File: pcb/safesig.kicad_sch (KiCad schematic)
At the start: 6 parts, among them U7 74HC123

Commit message: Add LCSCs.
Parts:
- R27, R28: LCSC (none) -> C17713
- U7: LCSC (none) -> C91435
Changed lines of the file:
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@@
+      (effects (font (size 1.27 1.27)) hide)
+    )
+    (property "LCSC" "C91435" (id 4) (at 92.075 65.405 0)
       (effects (font (size 1.27 1.27)) hide)
     )
@@
       (effects (font (size 1.27 1.27)) hide)
     )
+    (property "LCSC" "C91435" (id 4) (at 92.075 120.65 0)
+      (effects (font (size 1.27 1.27)) hide)
+    )
     (pin "1")
     (pin "13")
@@
       (effects (font (size 1.27 1.27)) hide)
     )
+    (property "LCSC" "C17713" (id 4) (at 69.85 49.53 0)
+      (effects (font (size 1.27 1.27)) hide)
+    )
     (pin "1")
     (pin "2")
@@
       (effects (font (size 1.27 1.27)) hide)
     )
+    (property "LCSC" "C17713" (id 4) (at 69.85 104.775 0)
+      (effects (font (size 1.27 1.27)) hide)
+    )
     (pin "1")
     (pin "2")
@@
       (effects (font (size 1.27 1.27)) hide)
     )
+    (property "LCSC" "C91435" (id 4) (at 231.14 91.44 0)
+      (effects (font (size 1.27 1.27)) hide)
+    )

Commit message: Tweak silkscreen.
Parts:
- U7: JLCPCB_CORRECTION (none) -> 0;0;270
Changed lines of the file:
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@@
+      (effects (font (size 1.27 1.27)) hide)
+    )
+    (property "JLCPCB_CORRECTION" "0;0;270" (id 5) (at 92.075 65.405 0)
       (effects (font (size 1.27 1.27)) hide)
     )
@@
       (effects (font (size 1.27 1.27)) hide)
     )
+    (property "JLCPCB_CORRECTION" "0;0;270" (id 5) (at 92.075 120.65 0)
+      (effects (font (size 1.27 1.27)) hide)
+    )
     (pin "1")
     (pin "13")
@@
       (effects (font (size 1.27 1.27)) hide)
     )
+    (property "JLCPCB_CORRECTION" "0;0;270" (id 5) (at 231.14 91.44 0)
+      (effects (font (size 1.27 1.27)) hide)
+    )

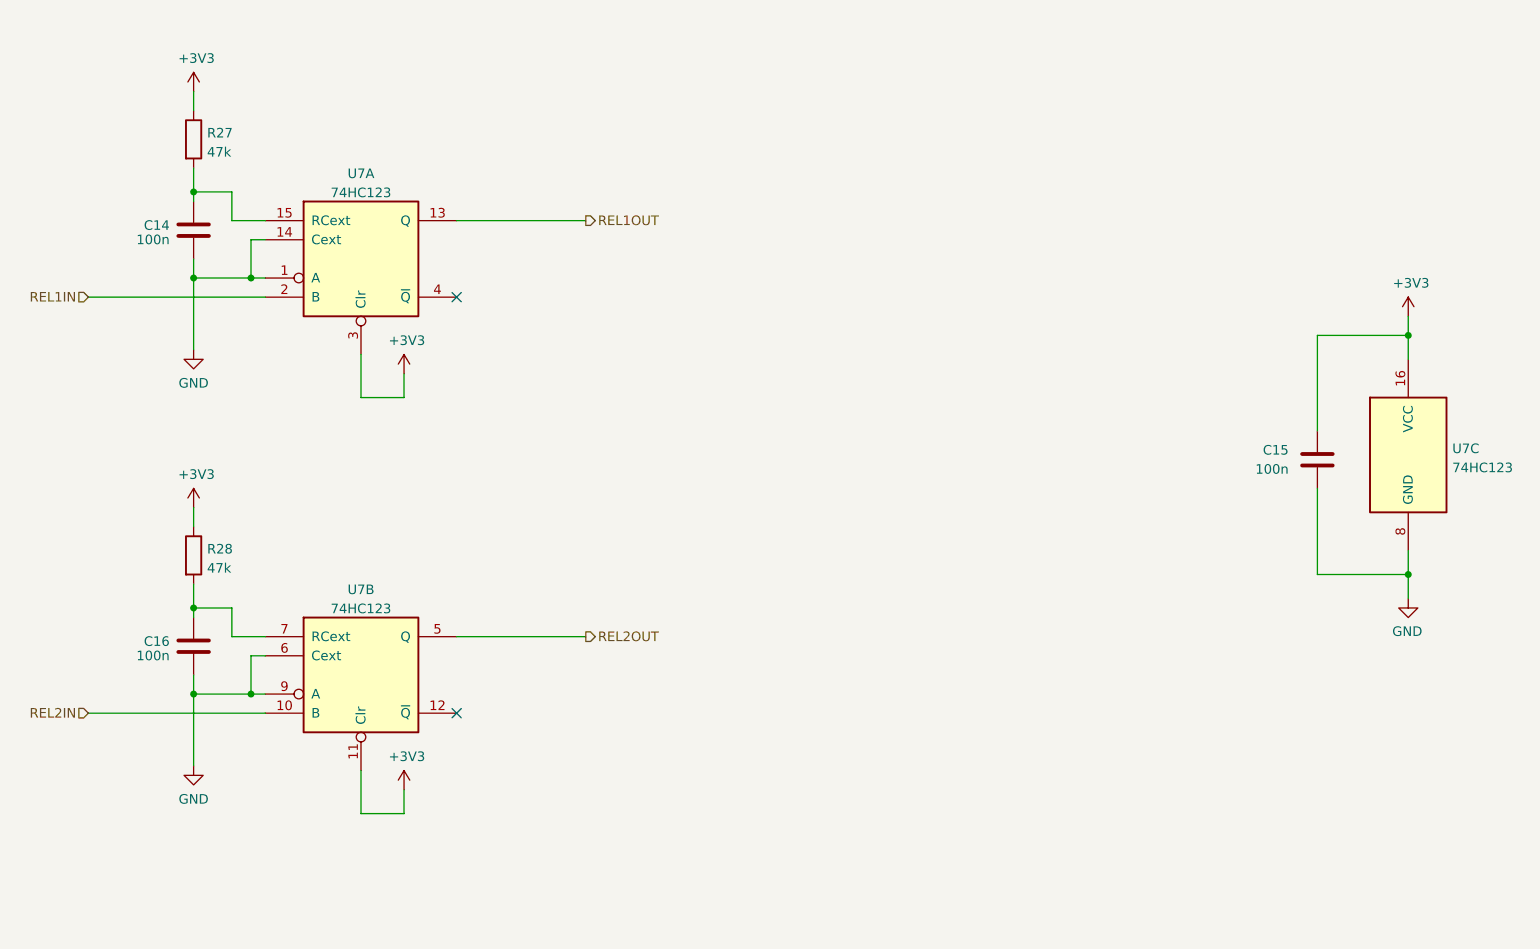
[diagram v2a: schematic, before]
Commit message: Add pull-down resistors to relay logic signals.
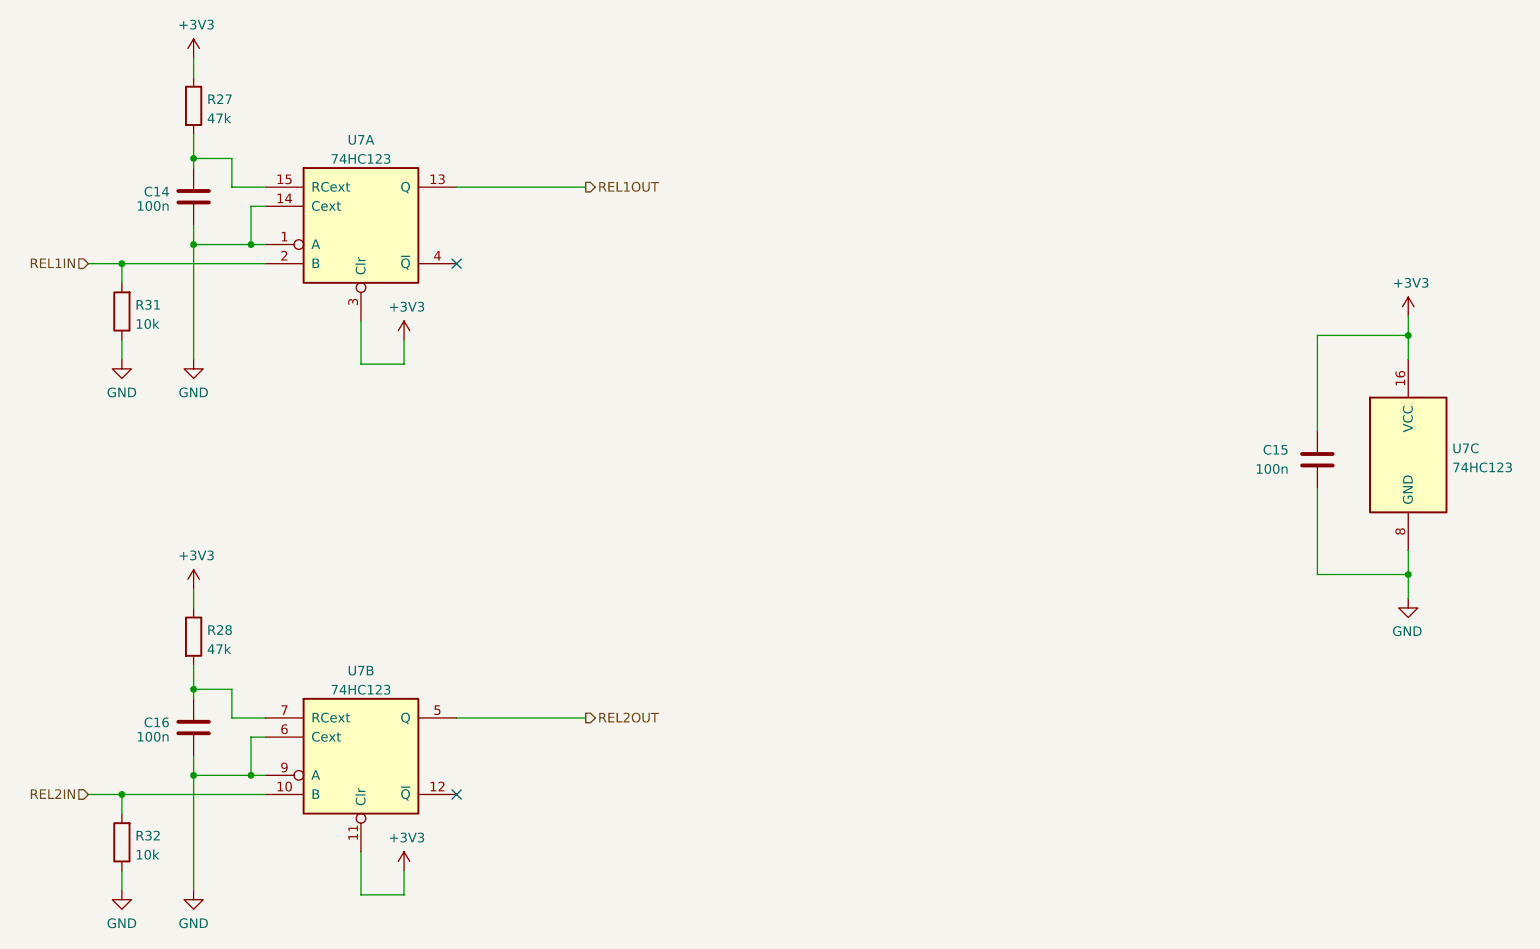
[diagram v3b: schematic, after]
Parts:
- added R31, R32: 10k, Resistor_SMD:R_0805_2012Metric, symbol Device:R
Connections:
- net GND: now also R31.1, R32.1
- net REL1IN: now also R31.2
- net REL2IN: now also R32.2
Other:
- moved on the sheet: C14, C16, R27, R28, U7A, U7B
